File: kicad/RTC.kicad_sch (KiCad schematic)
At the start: 16 parts, among them J9 Conn_01x02_Pin, Q6 PMOS, U7 PCF8523T, Y2 ABS07AIG-32.768KHZ-7-T

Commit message: layout floorplanning
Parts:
- C23, C24, C25: footprint Capacitor_SMD:C_0805_2012Metric_Pad1.18x1.45mm_HandSolder -> Capacitor_SMD:C_0603_1608Metric_Pad1.08x0.95mm_HandSolder; Package 0805 -> 0603
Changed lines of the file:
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@@
 			)
 		)
-		(property "Footprint" "Capacitor_SMD:C_0805_2012Metric_Pad1.18x1.45mm_HandSolder"
+		(property "Footprint" "Capacitor_SMD:C_0603_1608Metric_Pad1.08x0.95mm_HandSolder"
 			(at 119.38 92.4052 0)
 			(effects
@@
 			)
 		)
-		(property "Package" "0805"
+		(property "Package" "0603"
 			(at 123.19 91.44 90)
 			(effects
@@
 			)
 		)
-		(property "Footprint" "Capacitor_SMD:C_0805_2012Metric_Pad1.18x1.45mm_HandSolder"
+		(property "Footprint" "Capacitor_SMD:C_0603_1608Metric_Pad1.08x0.95mm_HandSolder"
 			(at 135.5852 66.04 0)
 			(effects
@@
 			)
 		)
-		(property "Package" "0805"
+		(property "Package" "0603"
 			(at 134.62 62.23 0)
 			(effects
@@
 			)
 		)
-		(property "Footprint" "Capacitor_SMD:C_0805_2012Metric_Pad1.18x1.45mm_HandSolder"
+		(property "Footprint" "Capacitor_SMD:C_0603_1608Metric_Pad1.08x0.95mm_HandSolder"
 			(at 145.7452 66.04 0)
 			(effects
@@
 			)
 		)
-		(property "Package" "0805"
+		(property "Package" "0603"
 			(at 144.78 62.23 0)
 			(effects

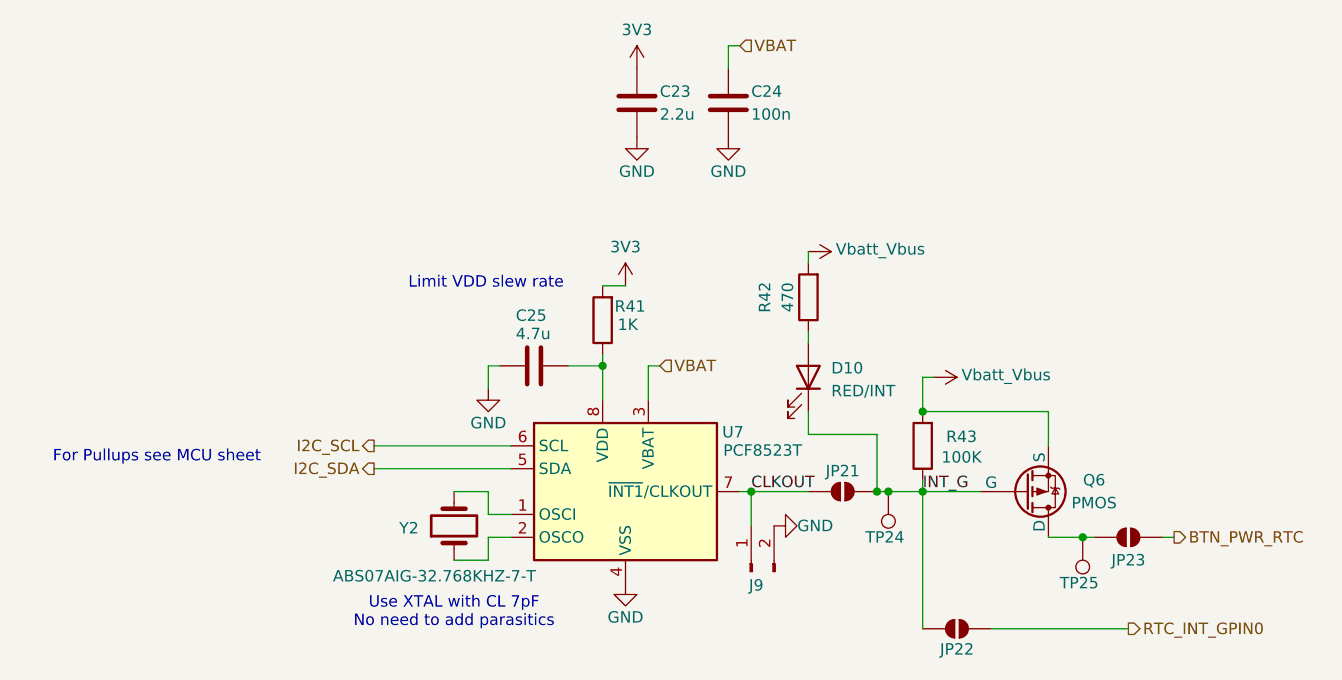
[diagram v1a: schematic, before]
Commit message: layout rtc
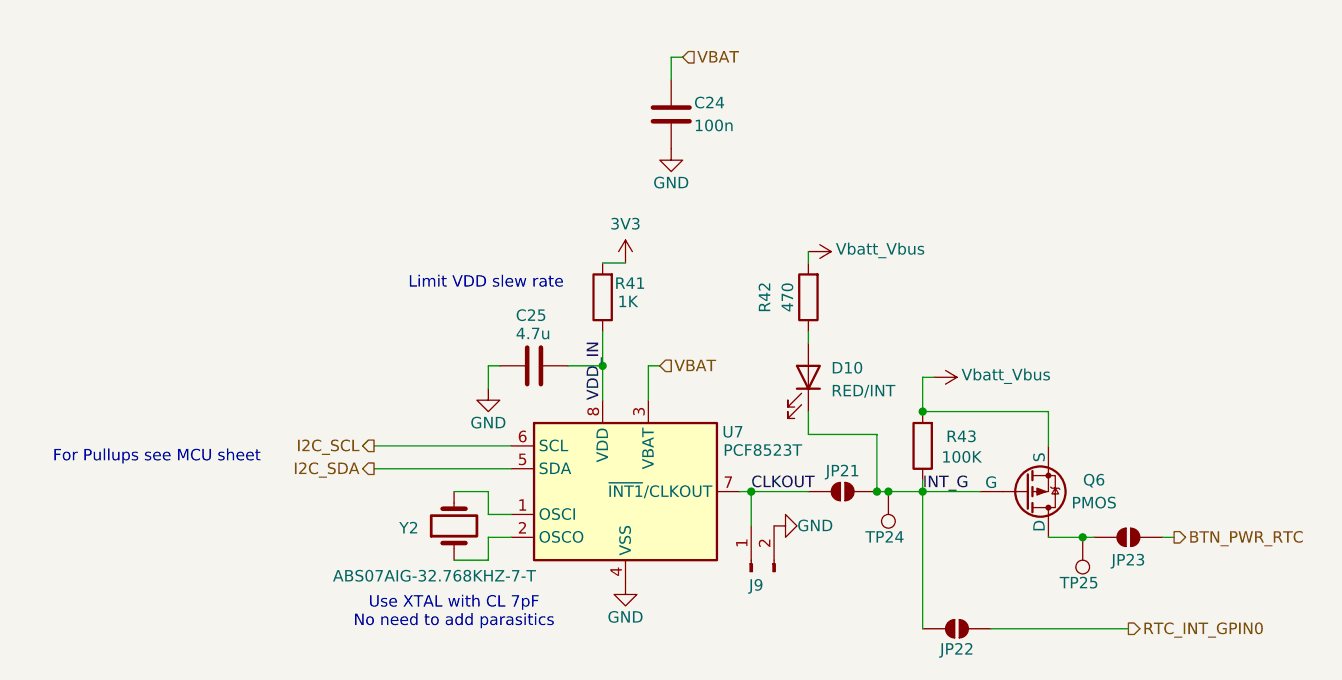
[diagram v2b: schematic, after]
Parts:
- removed C23: 2.2u, Capacitor_SMD:C_0603_1608Metric_Pad1.08x0.95mm_HandSolder, symbol Device:C
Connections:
- net VDD_IN: now reaches C25.1, R41.1, U7.8 (VDD)
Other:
- moved on the sheet: C24, R41
